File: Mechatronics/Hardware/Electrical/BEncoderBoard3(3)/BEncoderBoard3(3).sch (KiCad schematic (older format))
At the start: 8 parts, among them J1 Conn_01x04_Male, U8 RN4871U

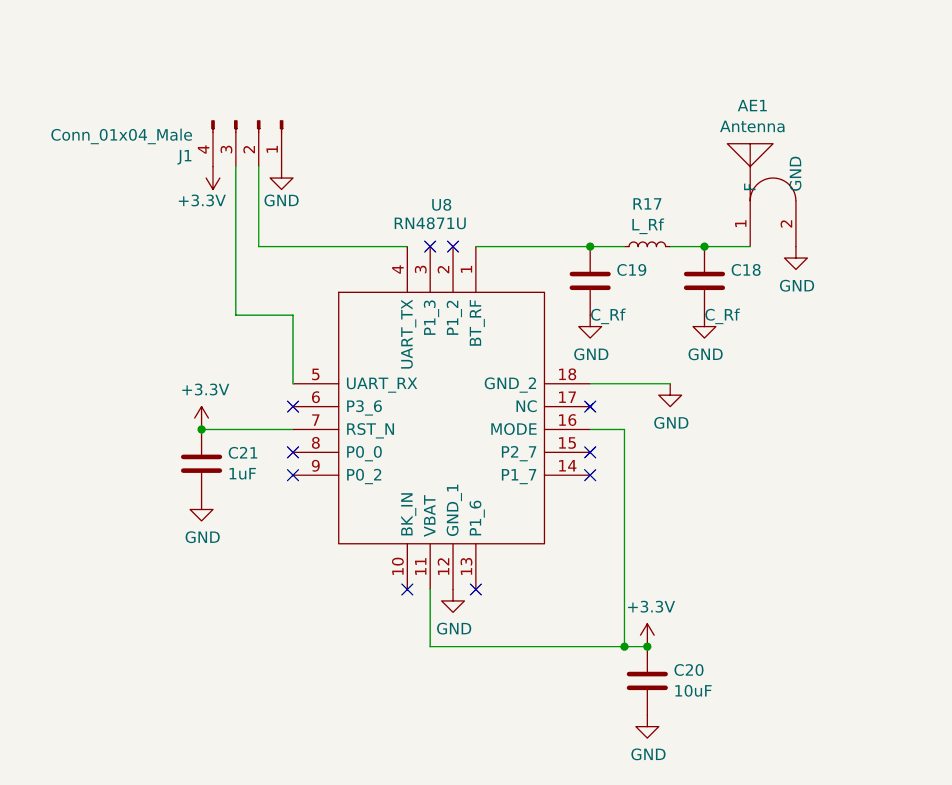
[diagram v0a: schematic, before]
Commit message: PCB changes
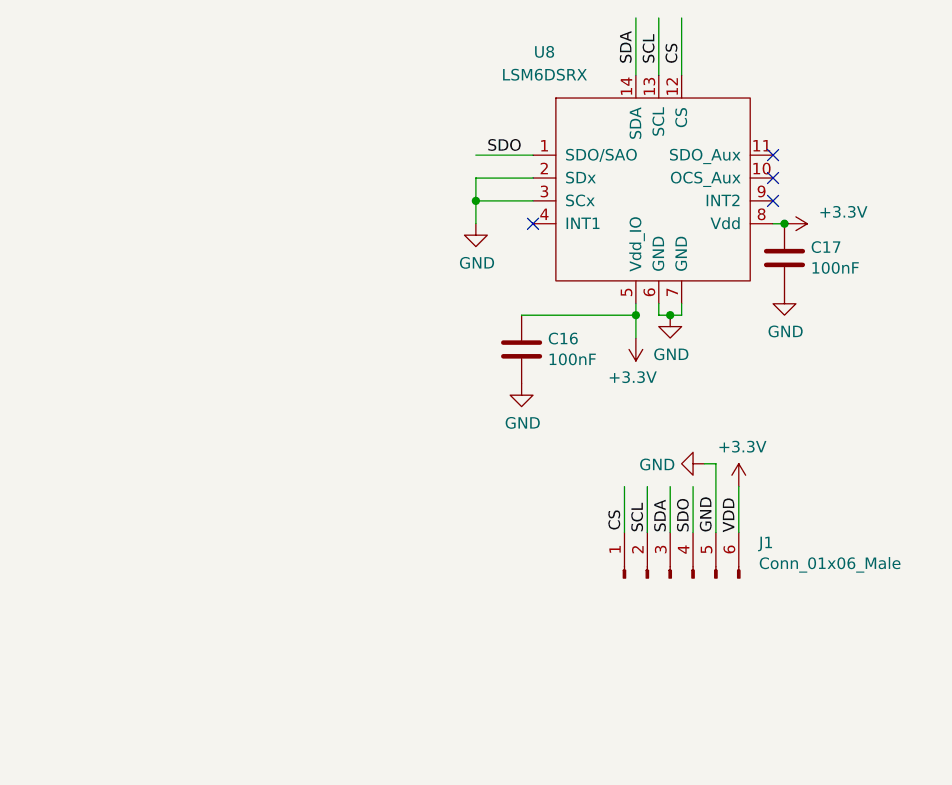
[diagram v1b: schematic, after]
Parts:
- removed AE1: Antenna, Encoder:Antenna, symbol Encoder:Antenna
- removed C18, C19: C_Rf, Encoder:C_0402_1005Metric, symbol Device:C
- removed C20: 10uF, Encoder:C_0603_1608Metric_Pad1.05x0.95mm_HandSolder, symbol Device:C
- removed C21: 1uF, Encoder:C_0603_1608Metric_Pad1.05x0.95mm_HandSolder, symbol Device:C
- removed J1: Conn_01x04_Male, Encoder:SolderWirePad_1x04_SMD_5x10mm_copy, symbol Connector:Conn_01x04_Male
- removed R17: L_Rf, Encoder:L_0402_1005Metric, symbol Device:L_Small
- removed U8: RN4871U, Encoder:RN4871U, symbol Encoder:RN4871U
- added C16, C17: 100nF, Encoder:C_0603_1608Metric_Pad1.05x0.95mm_HandSolder, symbol Device:C
- added J1: Conn_01x06_Male, Encoder:SolderWirePad_1x06_SMD_5x10mm, symbol Connector:Conn_01x06_Male
- added U8: LSM6DSRX, Encoder:LSM6DSRX, symbol Encoder:LSM6DSRX
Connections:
- net labels added: CS, SCL, SDA, SDO, VDD
- wire segments 16 -> 23
- no-connect marks 10 -> 4
